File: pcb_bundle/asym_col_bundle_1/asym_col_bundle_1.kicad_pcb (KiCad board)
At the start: 2 copper layers, 97.2 x 98.8 mm, 71 parts

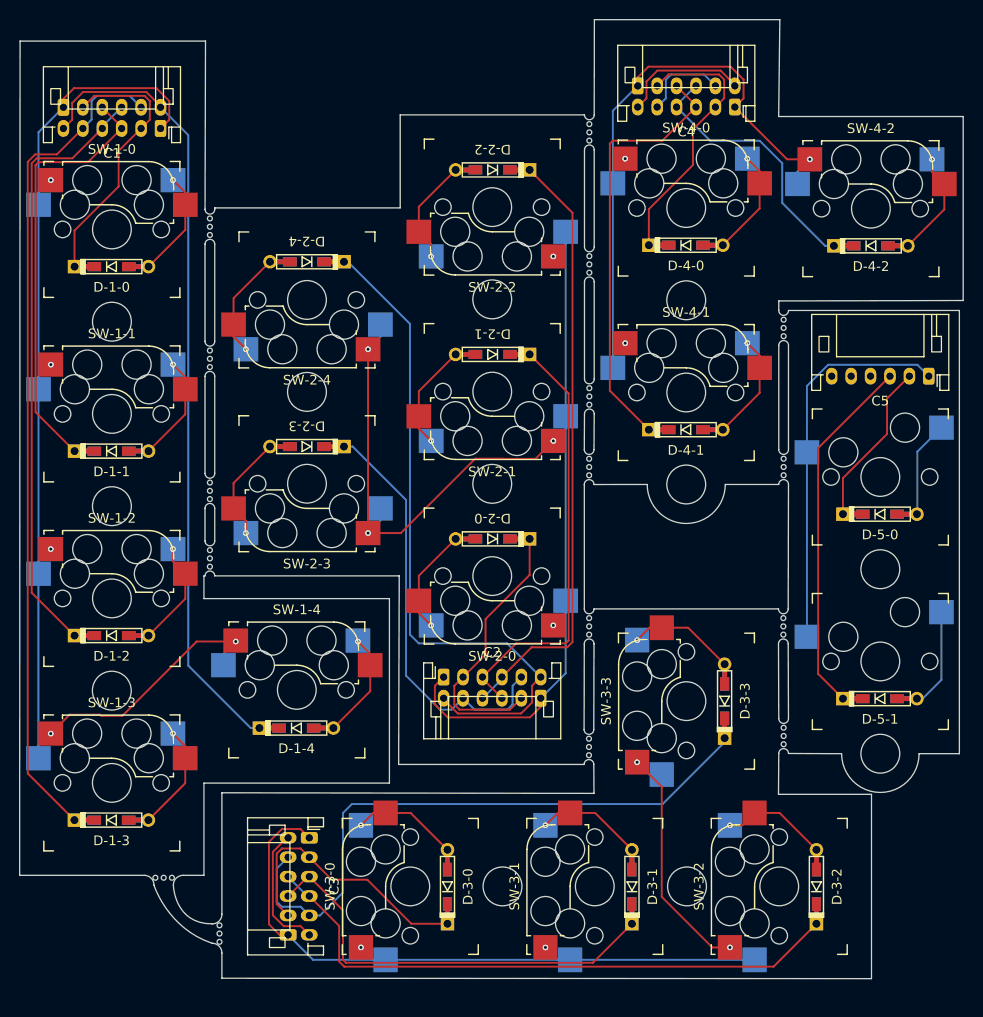
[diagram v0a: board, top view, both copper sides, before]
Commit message: [unstable] interim state
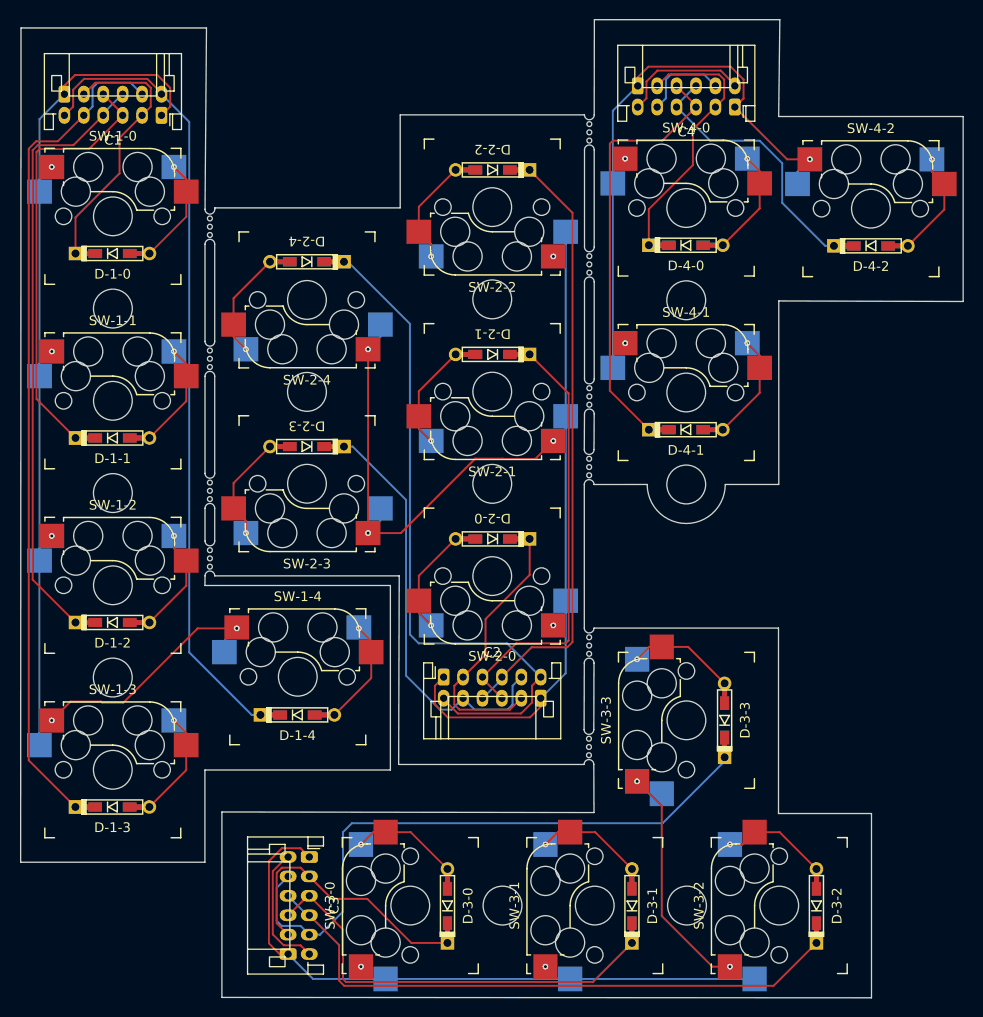
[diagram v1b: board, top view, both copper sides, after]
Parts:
- removed C5: Conn_01x06_Socket, Connector_JST:JST_PH_S6B-PH-K_1x06_P2.00mm_Horizontal
- removed D-5-0, D-5-1: D, crustrusk:Diode_TH_SMD_REVERSIBLE
- removed the REF** at (112.4, 125.3)
- removed the REF** at (54.5, 145.7)
- removed the REF** at (112.4, 83.3)
- removed the REF** at (112.4, 97.6)
- removed the REF** at (122.4, 127.2)
- removed the REF** at (122.4, 108.2)
- removed the REF** at (112.4, 114.1)
- removed the REF** at (48.5, 139.7)
- removed SW-5-0, SW-5-1: SW_Push, crustrusk:Kailh_socket_MX
- moved SW-3-0 1.97 mm to (73.9, 142.8)
- moved D-3-3 1.97 mm to (106.3, 123.7)
- moved C3 1.97 mm to (63.5, 137.8)
- moved D-3-0 1.97 mm to (77.8, 142.9)
- moved D-3-1 1.97 mm to (96.8, 142.9)
- moved D-3-2 1.97 mm to (115.8, 142.9)
- moved REF** 1.97 mm to (92.4, 116.0)
- moved REF** 1.97 mm to (83.4, 142.8)
- moved REF** 1.97 mm to (102.4, 142.8)
- moved SW-3-1 1.97 mm to (92.9, 142.8)
- moved SW-3-2 1.97 mm to (111.9, 142.8)
- moved SW-3-3 1.97 mm to (102.4, 123.7)
- moved SW-1-3 1.35 mm to (43.3, 128.8)
- moved D-1-2 1.35 mm to (43.3, 113.7)
- moved REF** 1.35 mm to (43.3, 100.3)
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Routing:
- net COL5: track 39.8 -> 0.00 mm
- net ROW1-5: track 37.3 -> 0.00 mm
- net ROW0-5: track 17.0 -> 0.00 mm
- net Net-(D-5-0-A): track 9.90 -> 0.00 mm
- net Net-(D-5-1-A): track 9.71 -> 0.00 mm
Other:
- board size 97.2 x 98.8 mm -> 97.1 x 100.7 mm
